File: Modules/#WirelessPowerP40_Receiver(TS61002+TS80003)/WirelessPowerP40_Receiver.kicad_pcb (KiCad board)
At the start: 4 copper layers, 53 x 53 mm, 162 parts, among them J1 Conn_01x02_Male, J2 I2C, J3 I2C, J4 I2C, J5 COIL 24uH, J6 Conn_01x02_Male, J7 Conn_01x02_Male, Q1 2N7002, Q2 2N7002, Q3 2N7002, Q4 2N7002, Q5 BSC100N06L, Q6 BSC028N06L, U1 TS30041, U2 TL431DBZ, U3 SC506, U4 TS61002, U5 TS80003, U6 IPG20N06S4L-11, U7 IPG20N06S4L-11, U8 max31740, U9 CSD16406Q3

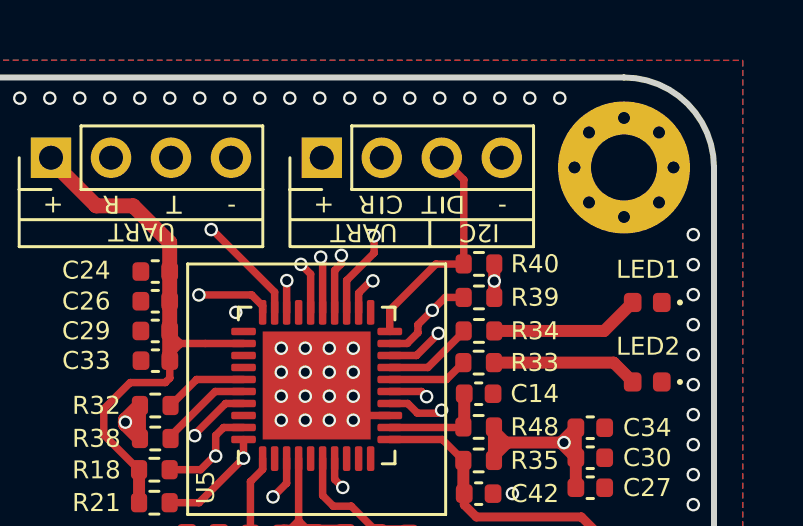
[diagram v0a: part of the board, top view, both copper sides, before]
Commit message: re-saved by kicad6
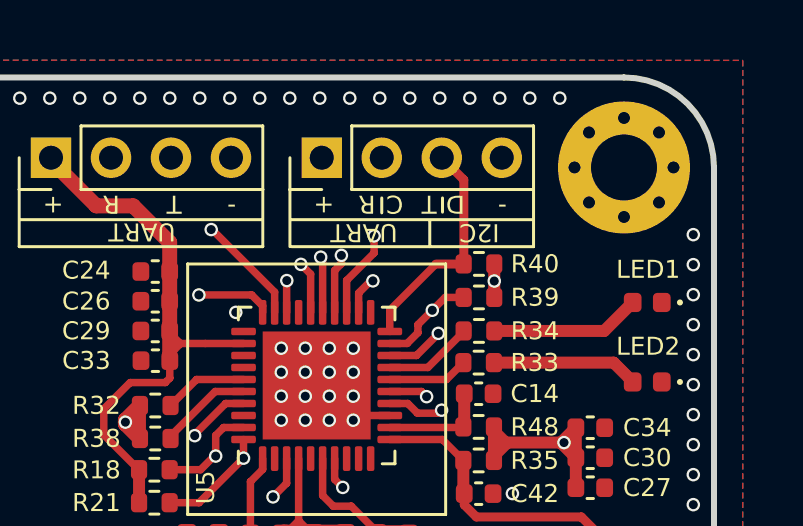
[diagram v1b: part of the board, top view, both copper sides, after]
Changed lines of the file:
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@@
   (net 64 "Net-(R25-Pad1)")
   (net 65 "Net-(D3-Pad3)")
-  (net 66 "Net-(R39-Pad2)")
+  (net 66 "Net-(J2-Pad2)")
   (net 67 "Net-(J2-Pad3)")
   (net 68 "Net-(J3-Pad2)")
@@
       (net 14 "+3V3") (pintype "passive"))
     (pad "2" smd roundrect locked (at 0.51 0 180) (size 0.54 0.64) (layers "F.Cu" "F.Paste" "F.Mask") (roundrect_rratio 0.25)
-      (net 66 "Net-(R39-Pad2)") (pintype "passive"))
+      (net 66 "Net-(J2-Pad2)") (pintype "passive"))
     (model "${KISYS3DMOD}/Resistor_SMD.3dshapes/R_0402_1005Metric.wrl"
       (offset (xyz 0 0 0))
@@
       (net 14 "+3V3") (pinfunction "Pin_1") (pintype "passive"))
     (pad "2" thru_hole oval locked (at 0 2 90) (size 1.35 1.35) (drill 0.8) (layers *.Cu *.Mask)
-      (net 66 "Net-(R39-Pad2)") (pinfunction "Pin_2") (pintype "passive"))
+      (net 66 "Net-(J2-Pad2)") (pinfunction "Pin_2") (pintype "passive"))
     (pad "3" thru_hole oval locked (at 0 4 90) (size 1.35 1.35) (drill 0.8) (layers *.Cu *.Mask)
       (net 67 "Net-(J2-Pad3)") (pinfunction "Pin_3") (pintype "passive"))
@@
       (net 102 "EN_DRV") (pinfunction "DRV_EN") (pintype "output"))
     (pad "19" smd roundrect locked (at 1.4 2.4375 90) (size 0.25 0.825) (layers "F.Cu" "F.Paste" "F.Mask") (roundrect_rratio 0.25)
-      (net 66 "Net-(R39-Pad2)") (pinfunction "I2C|SCL") (pintype "input"))
+      (net 66 "Net-(J2-Pad2)") (pinfunction "I2C|SCL") (pintype "input"))
     (pad "20" smd roundrect locked (at 1.8 2.4375 90) (size 0.25 0.825) (layers "F.Cu" "F.Paste" "F.Mask") (roundrect_rratio 0.25)
       (net 67 "Net-(J2-Pad3)") (pinfunction "I2C|SDA") (pintype "input"))
@@
   (segment (start 152.838214 75.831786) (end 153.455 75.831786) (width 0.25) (layer "F.Cu") (net 66))
   (via (at 152.41 76.26) (size 0.45) (drill 0.3) (layers "F.Cu" "B.Cu") (net 66))
-  (segment (start 152.41 76.26) (end 152.41 72.86) (width 0.25) (layer "In1.Cu") (net 66))
-  (segment (start 152.41 72.86) (end 150.725 71.175) (width 0.25) (layer "In1.Cu") (net 66))
+  (segment (start 152.41 76.26) (end 152.41 72.86) (width 0.3) (layer "In1.Cu") (net 66))
+  (segment (start 152.41 72.86) (end 150.725 71.175) (width 0.3) (layer "In1.Cu") (net 66))
   (segment (start 150.9925 76.967501) (end 150.9925 76.2575) (width 0.25) (layer "F.Cu") (net 67))
-  (segment (start 153.46 71.91) (end 153.46 74.71) (width 0.25) (layer "F.Cu") (net 67))
-  (segment (start 152.53 74.72) (end 153.47 74.72) (width 0.25) (layer "F.Cu") (net 67))
-  (segment (start 152.725 71.175) (end 153.46 71.91) (width 0.25) (layer "F.Cu") (net 67))
+  (segment (start 153.46 71.91) (end 153.46 74.71) (width 0.3) (layer "F.Cu") (net 67))
+  (segment (start 152.53 74.72) (end 153.47 74.72) (width 0.3) (layer "F.Cu") (net 67))
+  (segment (start 152.725 71.175) (end 153.46 71.91) (width 0.3) (layer "F.Cu") (net 67))
   (segment (start 150.9925 76.2575) (end 152.53 74.72) (width 0.25) (layer "F.Cu") (net 67))
   (segment (start 145.19 81.12) (end 145.14 81.12) (width 0.25) (layer "F.Cu") (net 68))
@@
   (segment (start 147.28 70.64) (end 146.57 69.93) (width 0.3) (layer "In2.Cu") (net 79))
   (segment (start 146.57 69.93) (end 131.84 69.93) (width 0.3) (layer "In2.Cu") (net 79))
-  (segment (start 131.84 69.93) (end 112.67 89.1) (width 0.3) (layer "In2.Cu") (net 79))
-  (segment (start 112.67 89.1) (end 112.67 105.42) (width 0.3) (layer "In2.Cu") (net 79))
+  (segment (start 131.84 69.93) (end 112.67 89.1) (width 0.5) (layer "In2.Cu") (net 79))
+  (segment (start 112.67 89.1) (end 112.67 105.42) (width 0.5) (layer "In2.Cu") (net 79))
   (segment (start 144.49 80.44) (end 144.49 80.4) (width 0.25) (layer "F.Cu") (net 80))
   (segment (start 145.522499 79.367501) (end 146.1175 79.367501) (width 0.25) (layer "F.Cu") (net 80))
